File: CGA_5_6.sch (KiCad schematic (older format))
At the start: 30 parts, among them Q1 2N3904, U13 74LS08, U14 74LS32, U15 74LS00, U20 74LS04, U21 74LS174, U24 74LS244, U41 74LS08, U42 74LS86, U43 74S74, U62 74LS125, U63 74LS175, U64 74LS164, U67 74LS244

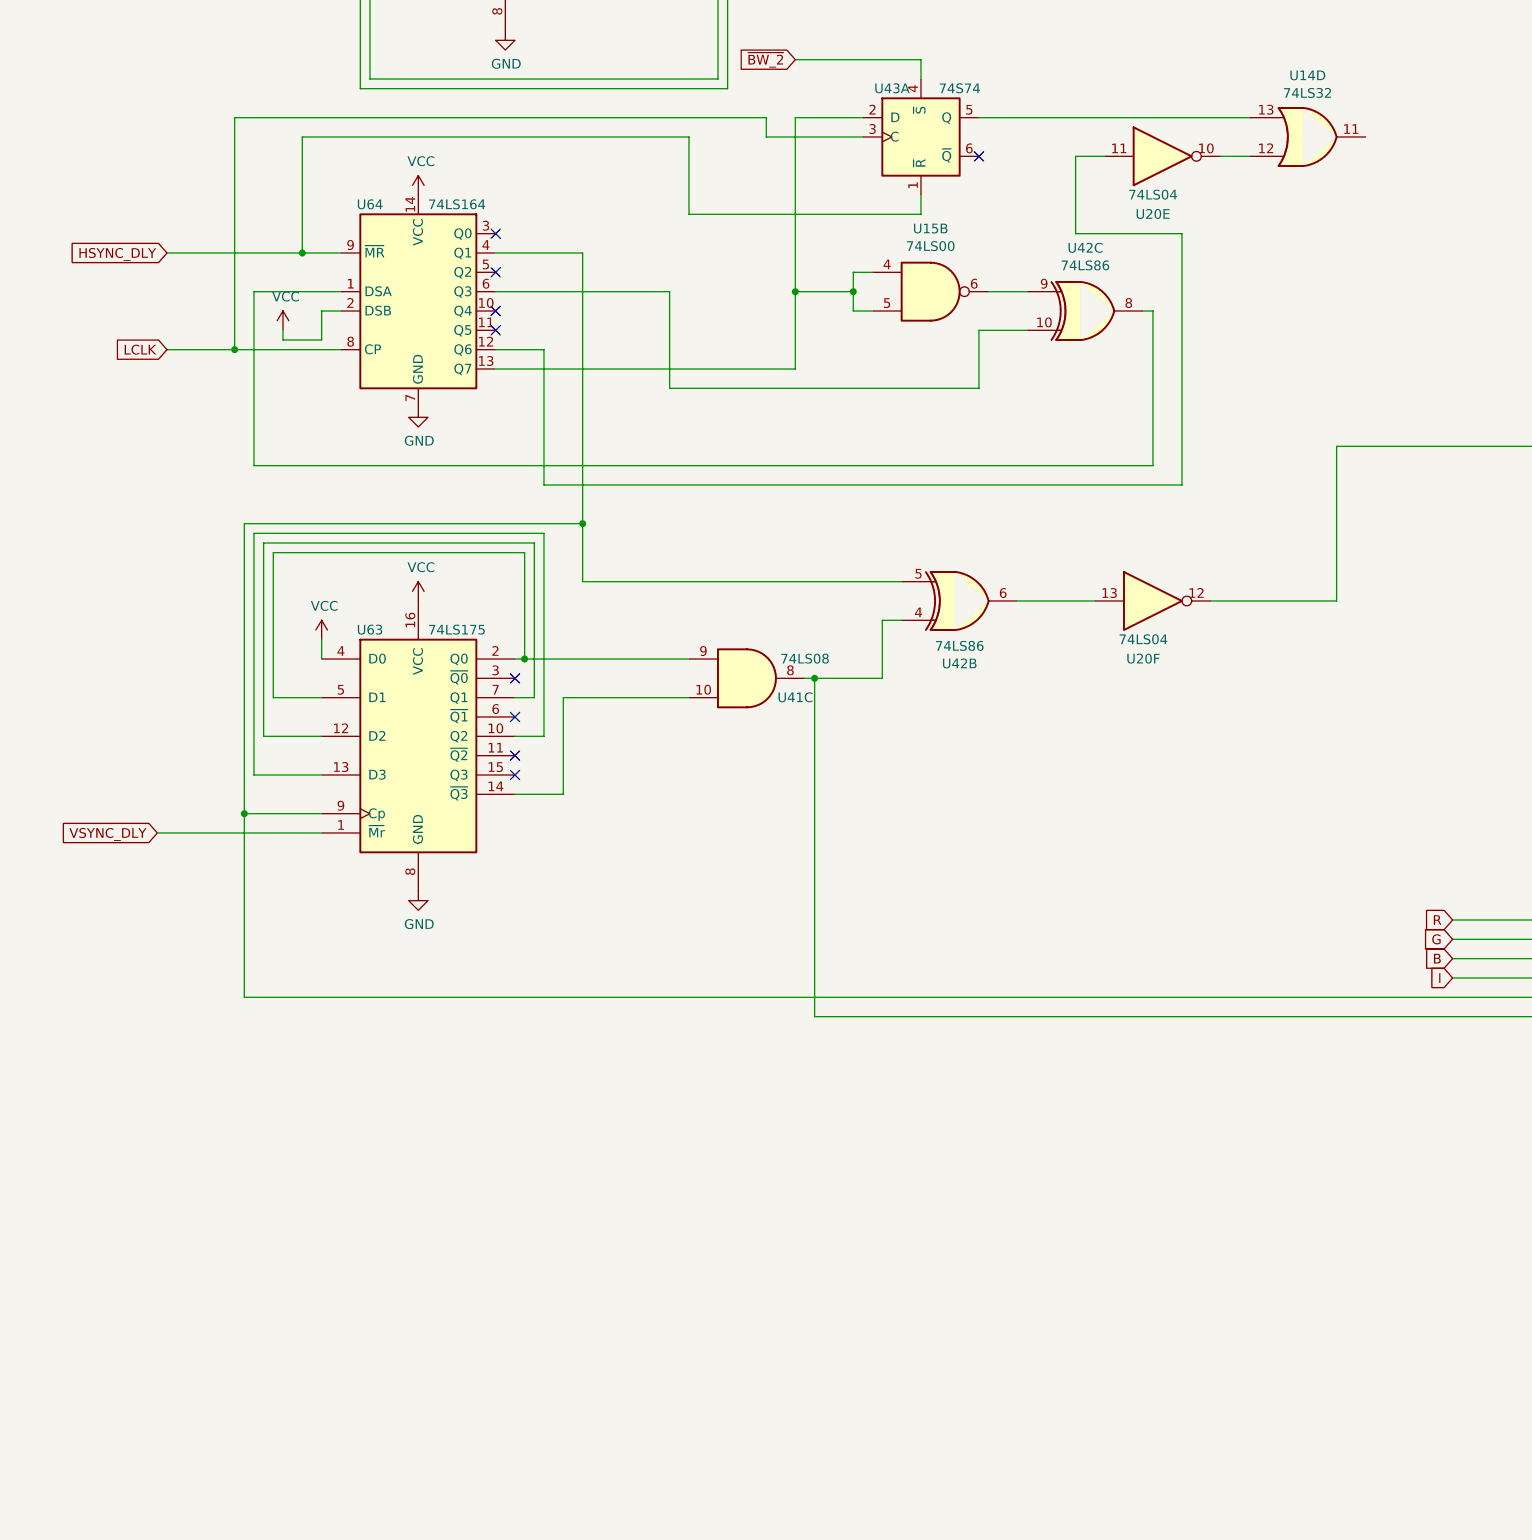
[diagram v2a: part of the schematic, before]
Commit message: More sheet 5
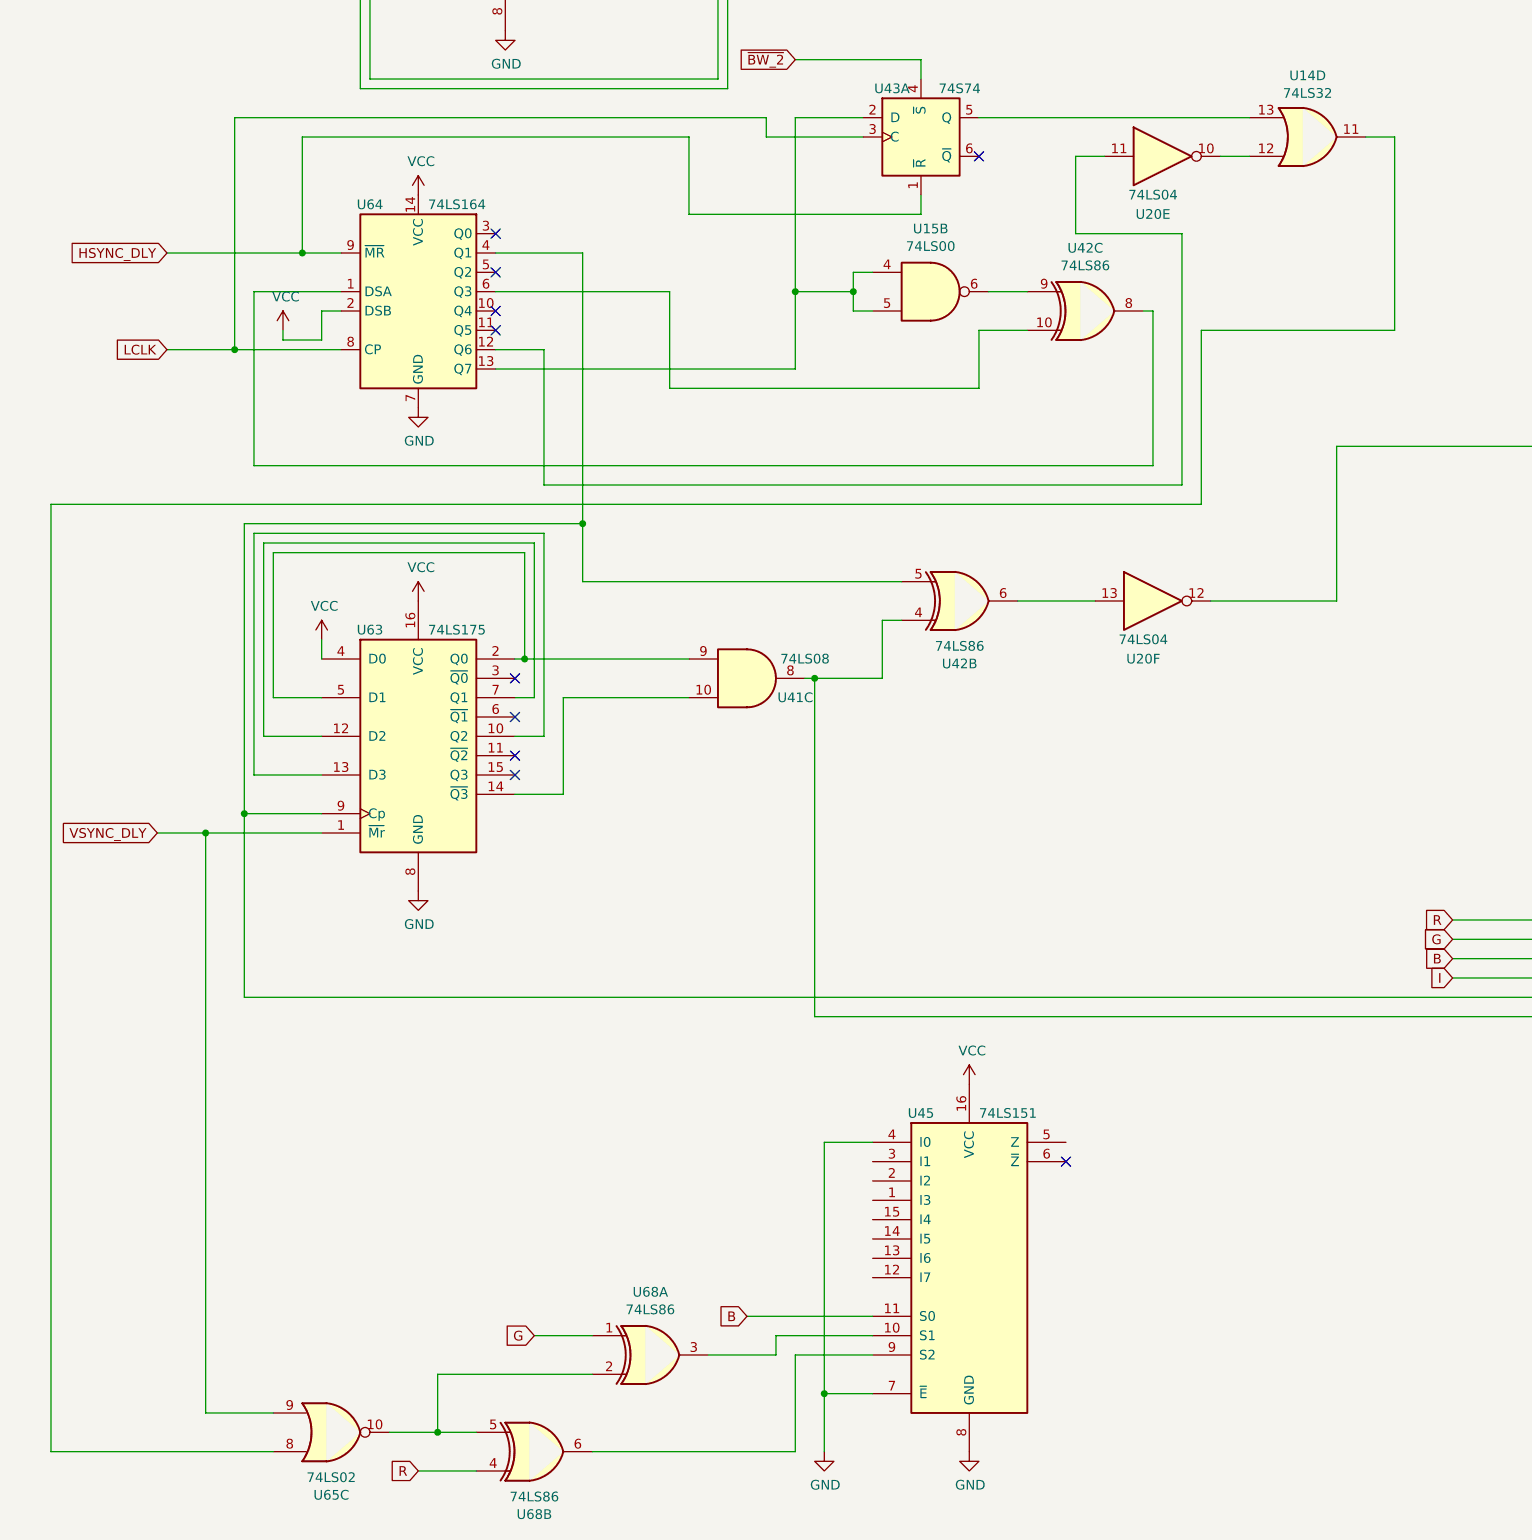
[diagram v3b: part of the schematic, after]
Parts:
- added U45: 74LS151, Package_DIP:DIP-16_W7.62mm_LongPads, symbol 74xx:74LS151
- added U65: 74LS02, Package_DIP:DIP-14_W7.62mm_LongPads, symbol 74xx:74LS02
- added U68: 74LS86, Package_DIP:DIP-14_W7.62mm_LongPads, symbol 74xx:74LS86
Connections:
- net B: now also U45.11 (S0)
- net G: now also U68.1
- net GND: now also U45.4 (I0), U45.7 (~E), U45.8 (GND)
- net R: now also U68.4
- net VCC: now also U45.16 (VCC)
- net VSYNC_DLY: now also U65.9
- net at U14.11: now also U65.8
- new net: U65.10, U68.2, U68.5
- new net: U45.9 (S2), U68.6
- new net: U45.10 (S1), U68.3
- no-connect marks 18 -> 19
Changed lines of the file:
@@
 VSYNC_DLY
-Wire Wire Line
-	1250 6850 2100 6850
 Wire Wire Line
 	3100 5950 3150 5950
@@
 Wire Wire Line
 	4650 6050 5000 6050
+$Comp
+L 74xx:74LS02 U?
+U 3 1 64443C3F
+P 2150 9950
+AR Path="/60463C57/64443C3F" Ref="U?"  Part="4"
+AR Path="/60463CF3/64443C3F" Ref="U65"  Part="3"
+F 0 "U65" H 2150 10275 50  0000 C CNN
+F 1 "74LS02" H 2150 10184 50  0000 C CNN
+F 2 "Package_DIP:DIP-14_W7.62mm_LongPads" H 2150 9950 50  0001 C CNN
+F 3 "http://www.ti.com/lit/gpn/sn74ls02" H 2150 9950 50  0001 C CNN
+	3    2150 9950
+	1    0    0    1
+$EndComp
+Wire Wire Line
+	1250 6850 1500 6850
+Wire Wire Line
+	1850 9850 1500 9850
+Connection ~ 1500 6850
+Wire Wire Line
+	1500 6850 2100 6850
+Wire Wire Line
+	7500 3250 7650 3250
+Wire Wire Line
+	7650 3250 7650 4250
+Wire Wire Line
+	7650 4250 6650 4250
+Wire Wire Line
+	6650 4250 6650 5150
+Wire Wire Line
+	700  5150 6650 5150
+Wire Wire Line
+	700  10050 1850 10050
+$Comp
+L 74xx:74LS86 U?
+U 2 1 644BB5C8
+P 3200 10050
+AR Path="/60463C10/644BB5C8" Ref="U?"  Part="4"
+AR Path="/60463CF3/644BB5C8" Ref="U68"  Part="2"
+F 0 "U68" H 3200 10375 50  0000 C CNN
+F 1 "74LS86" H 3200 10284 50  0000 C CNN
+F 2 "Package_DIP:DIP-14_W7.62mm_LongPads" H 3200 10050 50  0001 C CNN
+F 3 "74xx/74ls86.pdf" H 3200 10050 50  0001 C CNN
+	2    3200 10050
+	1    0    0    1
+$EndComp
+Wire Wire Line
+	2450 9950 2700 9950
+Text GLabel 2600 10150 0    50   Input ~ 0
+R
+Wire Wire Line
+	2600 10150 2900 10150
+$Comp
+L 74xx:74LS86 U?
+U 1 1 6450EEF8
+P 3800 9550
+AR Path="/60463C10/6450EEF8" Ref="U?"  Part="4"
+AR Path="/60463CF3/6450EEF8" Ref="U68"  Part="1"
+F 0 "U68" H 3800 9875 50  0000 C CNN
+F 1 "74LS86" H 3800 9784 50  0000 C CNN
+F 2 "Package_DIP:DIP-14_W7.62mm_LongPads" H 3800 9550 50  0001 C CNN
+F 3 "74xx/74ls86.pdf" H 3800 9550 50  0001 C CNN
+	1    3800 9550
+	1    0    0    -1
+$EndComp
+Wire Wire Line
+	3500 9650 2700 9650
+Wire Wire Line
+	2700 9650 2700 9950
+Connection ~ 2700 9950
+Wire Wire Line
+	2700 9950 2900 9950
+Text GLabel 3200 9450 0    50   Input ~ 0
+G
+Wire Wire Line
+	3200 9450 3500 9450
+$Comp
+L 74xx:74LS151 U45
+U 1 1 6455FCDF
+P 5450 9050
+F 0 "U45" H 5200 9800 50  0000 C CNN
+F 1 "74LS151" H 5650 9800 50  0000 C CNN
+F 2 "Package_DIP:DIP-16_W7.62mm_LongPads" H 5450 9050 50  0001 C CNN
+F 3 "http://www.ti.com/lit/gpn/sn74LS151" H 5450 9050 50  0001 C CNN
+	1    5450 9050
+	1    0    0    -1
+$EndComp
+$Comp
+L power:GND #PWR?
+U 1 1 64564397
+P 5450 10050
+F 0 "#PWR?" H 5450 9800 50  0001 C CNN
+F 1 "GND" H 5455 9877 50  0000 C CNN
+F 2 "" H 5450 10050 50  0001 C CNN
+F 3 "" H 5450 10050 50  0001 C CNN
+	1    5450 10050
+	1    0    0    -1
+$EndComp
+$Comp
+L power:VCC #PWR?
+U 1 1 64565099
+P 5450 8150
+F 0 "#PWR?" H 5450 8000 50  0001 C CNN
+F 1 "VCC" H 5465 8323 50  0000 C CNN
+F 2 "" H 5450 8150 50  0001 C CNN
+F 3 "" H 5450 8150 50  0001 C CNN
+	1    5450 8150
+	1    0    0    -1
+$EndComp
+NoConn ~ 5950 8550
+Wire Wire Line
+	1500 6850 1500 9850
+Wire Wire Line
+	700  5150 700  10050
+Wire Wire Line
+	3500 10050 4550 10050
+Wire Wire Line
+	4550 10050 4550 9550
+Wire Wire Line
+	4550 9550 4950 9550
+Wire Wire Line
+	4450 9550 4450 9450
+Wire Wire Line
+	4450 9450 4950 9450
+Wire Wire Line
+	4100 9550 4450 9550
+Text GLabel 4300 9350 0    50   Input ~ 0
+B
+Wire Wire Line
+	4300 9350 4950 9350
+Wire Wire Line
+	4950 8450 4700 8450
+Wire Wire Line
+	4700 8450 4700 9750
+Wire Wire Line
+	4950 9750 4700 9750
+Connection ~ 4700 9750
+Wire Wire Line
+	4700 9750 4700 10050
+$Comp
+L power:GND #PWR?
+U 1 1 6461E739
+P 4700 10050
+F 0 "#PWR?" H 4700 9800 50  0001 C CNN
+F 1 "GND" H 4705 9877 50  0000 C CNN
+F 2 "" H 4700 10050 50  0001 C CNN
+F 3 "" H 4700 10050 50  0001 C CNN
+	1    4700 10050
+	1    0    0    -1
+$EndComp
 $EndSCHEMATC

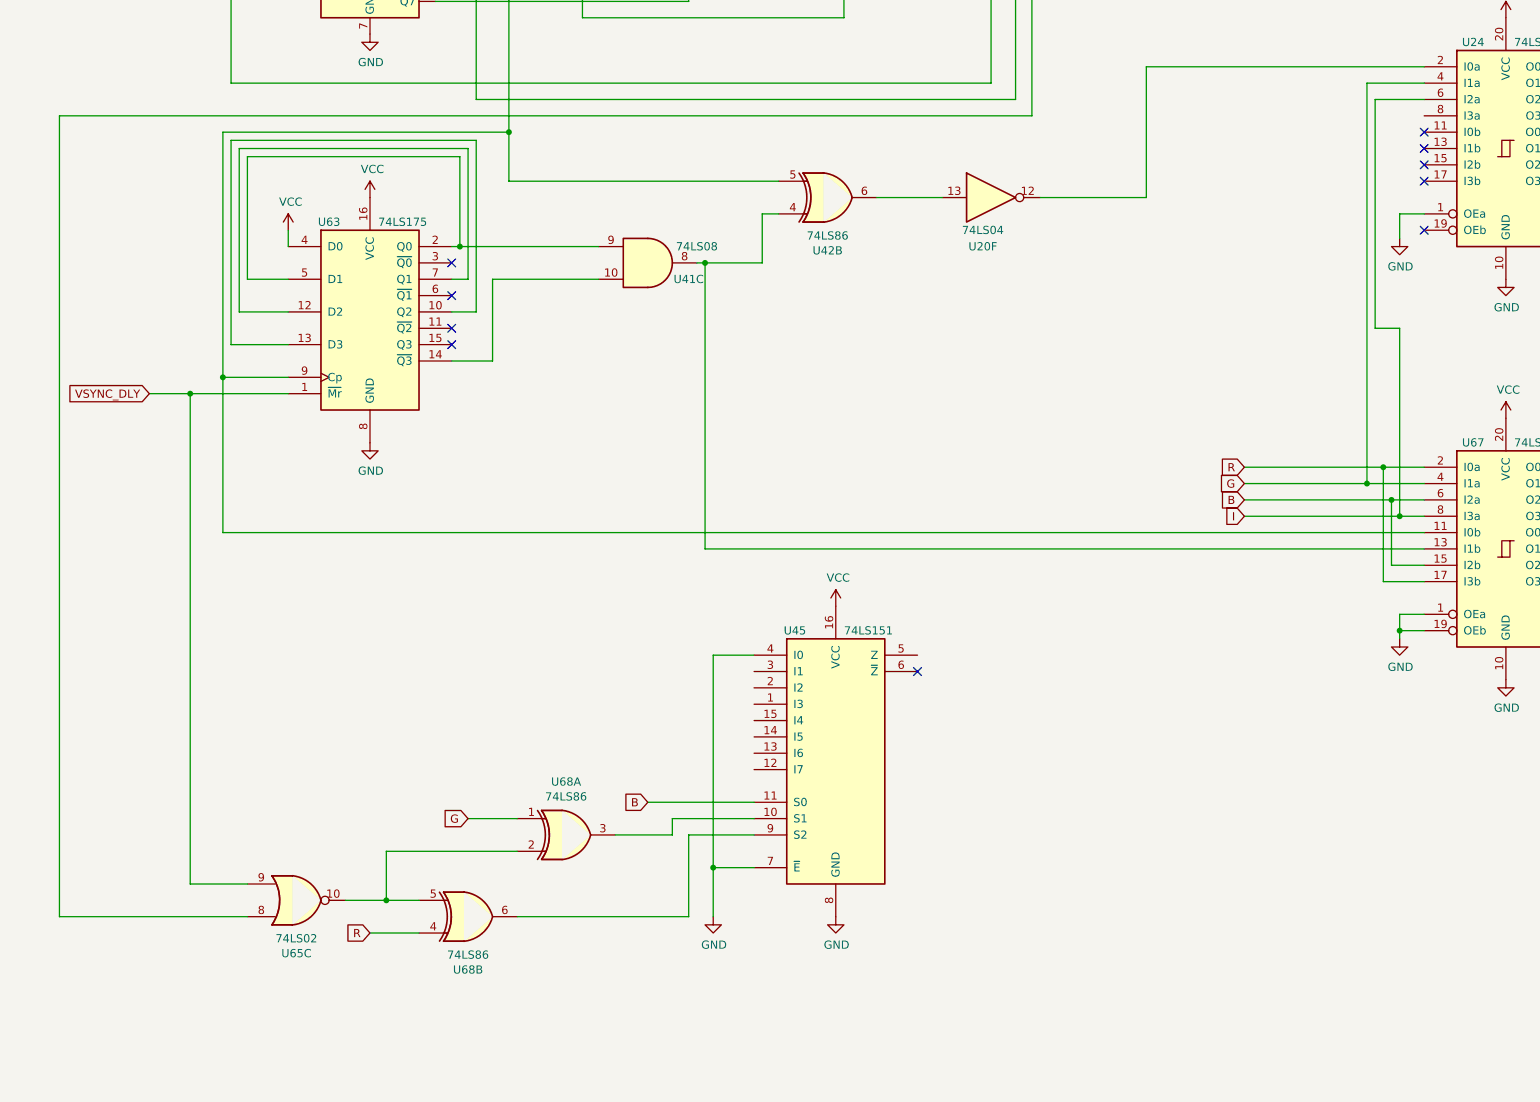
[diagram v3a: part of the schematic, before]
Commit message: More sheet 5
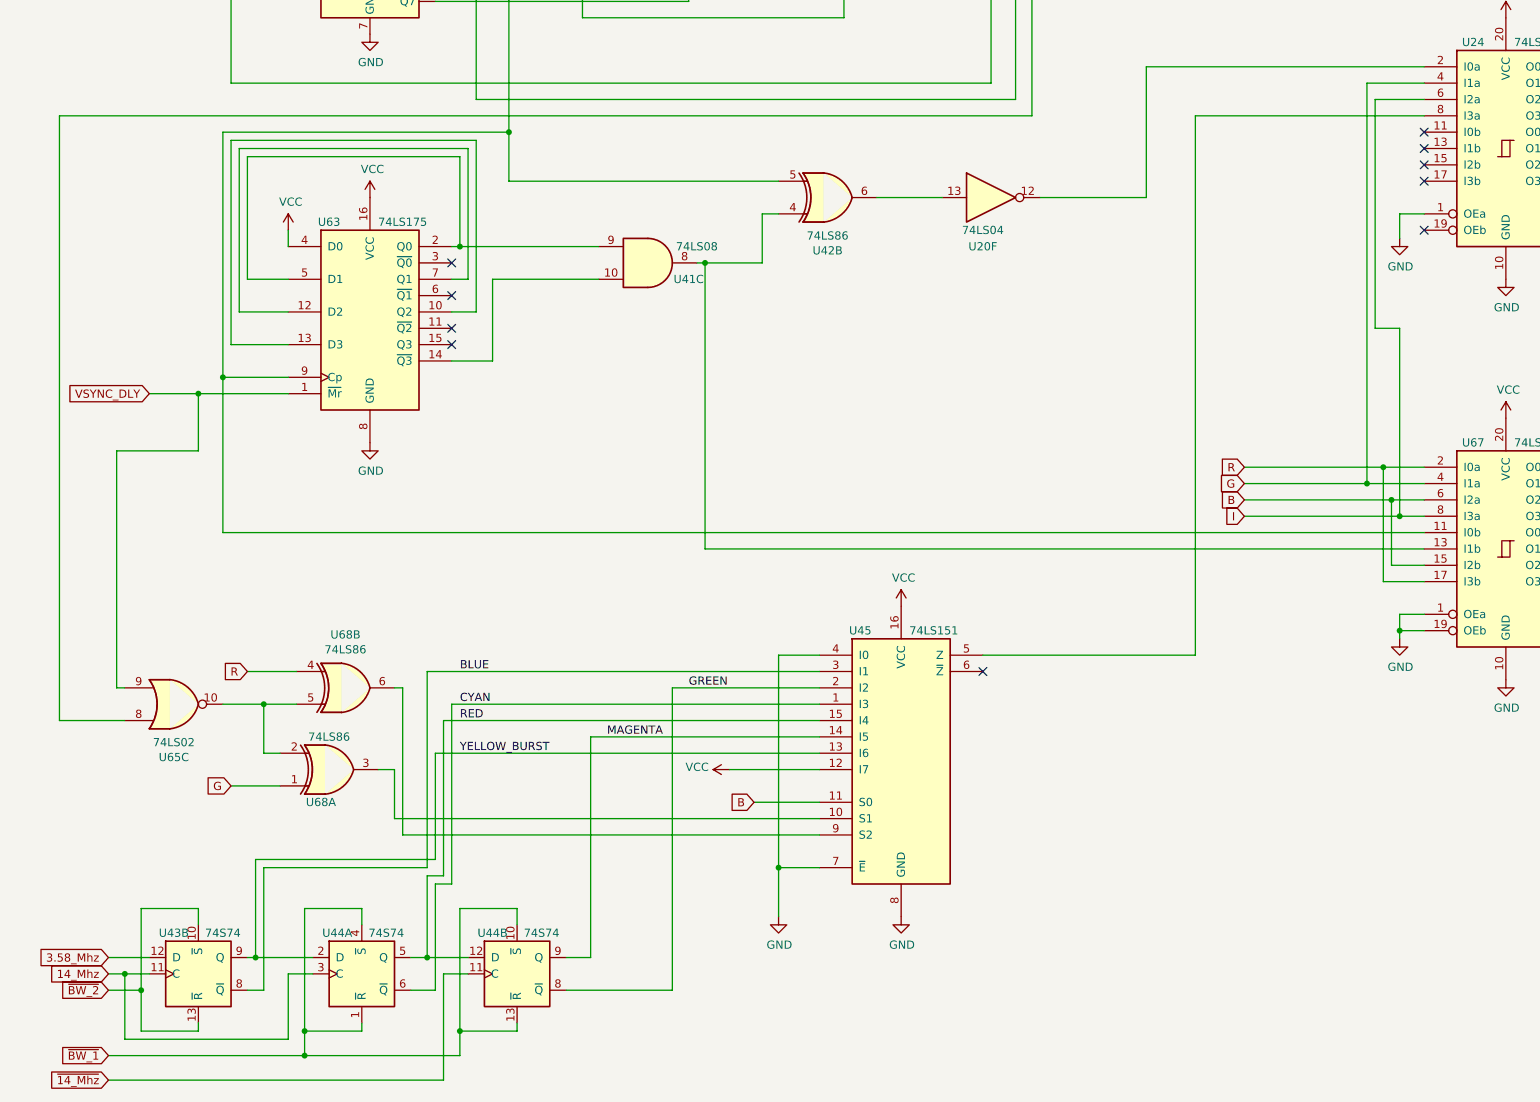
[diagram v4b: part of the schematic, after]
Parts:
- added unit 2 of U43
- added U44: 74S74, Package_DIP:DIP-14_W7.62mm_LongPads, symbol 74xx:74LS74
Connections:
- net VCC: now also U45.12 (I7)
- net ~BW_2: now also U43.10 (~S), U43.13 (~R)
- net at U24.8 (I3a): now also U45.5 (Z)
- net CYAN: now reaches U45.1 (I3)
- net CYAN: now also U44.6 (~Q)
- net YELLOW_BURST: now reaches U45.13 (I6)
- net YELLOW_BURST: now also U43.9 (Q), U44.2 (D)
- net MAGENTA: now reaches U45.14 (I5)
- net MAGENTA: now also U44.9 (Q)
- net RED: now reaches U45.15 (I4)
- net RED: now also U44.12 (D), U44.5 (Q)
- net GREEN: now reaches U45.2 (I2)
- net GREEN: now also U44.8 (~Q)
- net BLUE: now reaches U45.3 (I1)
- net BLUE: now also U43.8 (~Q)
- new net 14_Mhz: U43.11 (C), U44.3 (C)
- new net 3.58_Mhz: U43.12 (D)
- new net ~14_Mhz: U44.11 (C)
- new net ~BW_1: U44.1 (~R), U44.10 (~S), U44.13 (~R), U44.4 (~S)
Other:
- moved on the sheet: U45, U65C, U68A, U68B
